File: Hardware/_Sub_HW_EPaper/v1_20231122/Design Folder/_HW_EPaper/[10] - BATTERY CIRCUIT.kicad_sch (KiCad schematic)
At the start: 0 parts

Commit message: Working on E-Paper schematic
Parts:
- added C1001, C1003: 1uF_10V_X7R, Capacitor_SMD:C_0402_1005Metric, symbol _SCHLIB_Epaper:CAP_1uF_10V_X7R_C0402
- added C1002, C1004: 100nF_50V, Capacitor_SMD:C_0402_1005Metric, symbol _SCHLIB_Epaper:CAP_100nF_50V_X7R_C0402
- added R1001: 10kR_1/16W_1%, Resistor_SMD:R_0402_1005Metric, symbol _SCHLIB_Epaper:RES_10kR_1/16W_1%_R0402
- added U1001: NCP551SN33T1G, Package_SO:TSOP-5_1.65x3.05mm_P0.95mm, symbol _SCHLIB_Epaper:PMIC_LDO_NCP551SN33T1G_+3V3DC_150mA_5-TSOP
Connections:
- new net: C1001.1, C1002.1, R1001.1, U1001.1 (VIN)
- new net +3V3: C1003.1, C1004.1, U1001.5 (VOUT)
- new net GND: C1001.2, C1002.2, C1003.2, C1004.2, U1001.2 (GND)
- new net NCP551_EN: R1001.2, U1001.3 (ENABLE)
- no-connect marks 0 -> 1

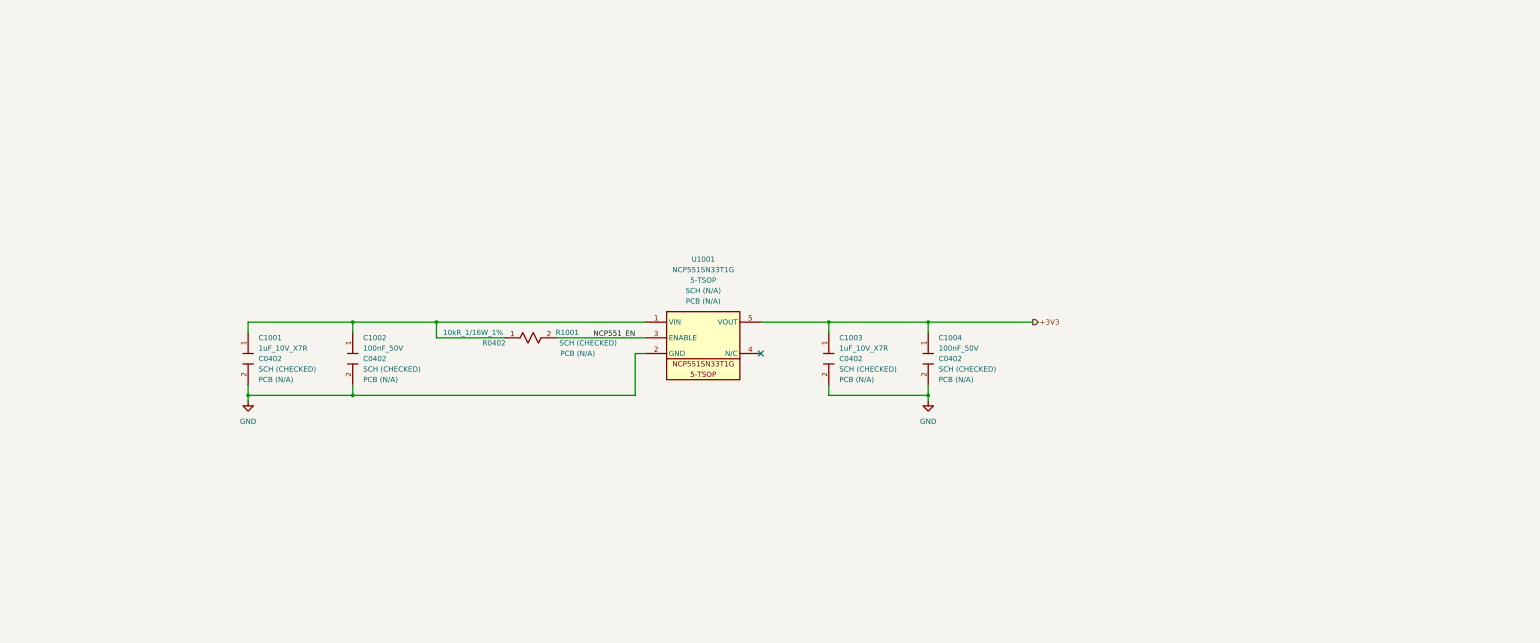
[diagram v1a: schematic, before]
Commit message: EPaper schematic is almost done...
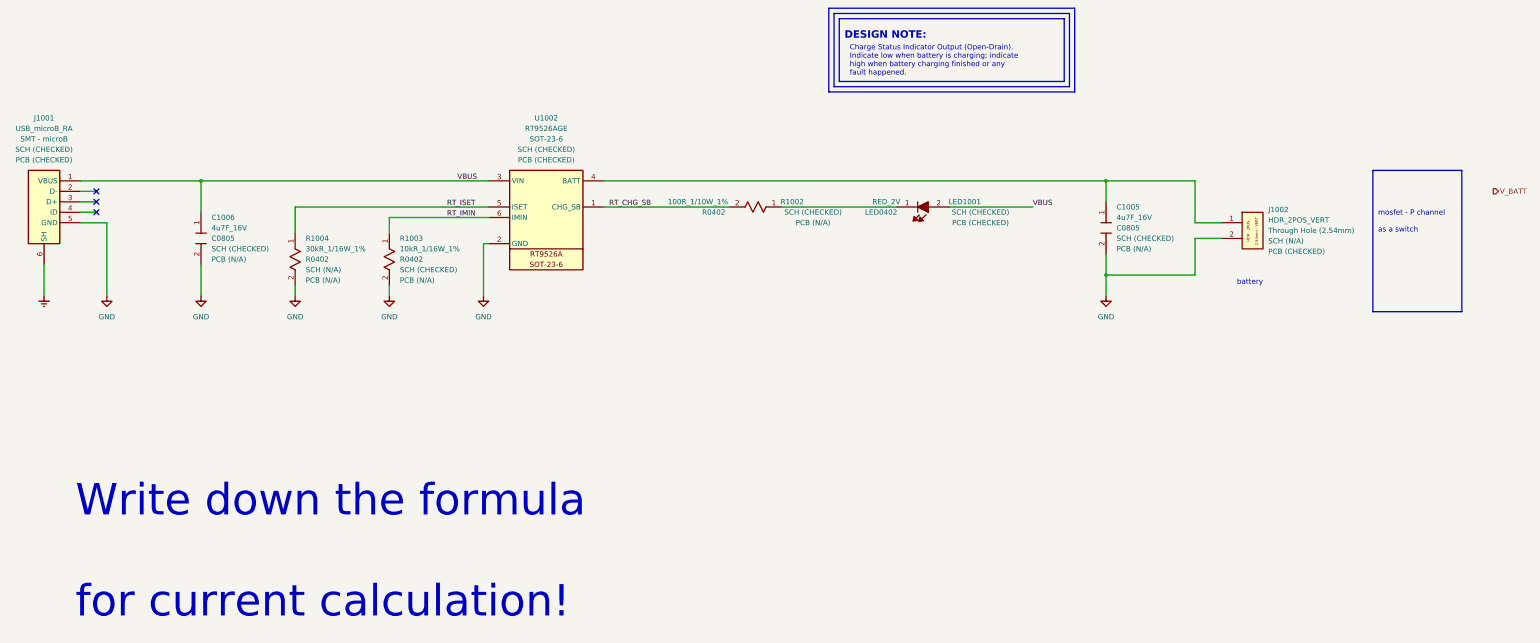
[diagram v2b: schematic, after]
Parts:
- removed C1001, C1003: 1uF_10V_X7R, Capacitor_SMD:C_0402_1005Metric, symbol _SCHLIB_Epaper:CAP_1uF_10V_X7R_C0402
- removed C1002, C1004: 100nF_50V, Capacitor_SMD:C_0402_1005Metric, symbol _SCHLIB_Epaper:CAP_100nF_50V_X7R_C0402
- removed R1001: 10kR_1/16W_1%, Resistor_SMD:R_0402_1005Metric, symbol _SCHLIB_Epaper:RES_10kR_1/16W_1%_R0402
- removed U1001: NCP551SN33T1G, Package_SO:TSOP-5_1.65x3.05mm_P0.95mm, symbol _SCHLIB_Epaper:PMIC_LDO_NCP551SN33T1G_+3V3DC_150mA_5-TSOP
- added C1005, C1006: 4u7F_16V, Capacitor_SMD:C_0805_2012Metric, symbol _SCHLIB_Epaper:CAP_4.7uF_16V_X7R_C0805
- added J1001: USB_microB_RA, Connector_USB:USB_Micro-B_Amphenol_10118194_Horizontal, symbol _SCHLIB_Epaper:CONN_RECEPT_USB2.0_microB_5POS_RA
- added J1002: HDR_2POS_VERT, Connector_PinHeader_2.54mm:PinHeader_1x02_P2.54mm_Vertical, symbol _SCHLIB_Epaper:CONN_HEADER_2POS_1ROW_VERT_2.54mm
- added LED1001: RED_2V, LED_SMD:LED_0402_1005Metric, symbol _SCHLIB_Epaper:LED_RED_2V_624nm_LED0402
- added R1002: 100R_1/10W_1%, Resistor_SMD:R_0402_1005Metric, symbol _SCHLIB_Epaper:RES_100R_1/10W_1%_R0402
- added R1003: 10kR_1/16W_1%, Resistor_SMD:R_0402_1005Metric, symbol _SCHLIB_Epaper:RES_10kR_1/16W_1%_R0402
- added R1004: 30kR_1/16W_1%, Resistor_SMD:R_0402_1005Metric, symbol _SCHLIB_Epaper:RES_30kR_1/16W_1%_R0402
- added U1002: RT9526AGE, Package_TO_SOT_SMD:SOT-23-6, symbol _SCHLIB_Epaper:PMIC_CHARGER_RT9526AGE_LithiumIon_1C_SOT-23-6
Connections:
- net GND: now also C1005.2, C1006.2, J1001.5 (GND), J1002.2, R1003.2, R1004.2, U1002.2 (GND)
- new net: C1005.1, J1002.1, U1002.4 (BATT)
- new net: LED1001.1, R1002.1
- new net Earth: J1001.6 (SH)
- new net RT_CHG_SB: R1002.2, U1002.1 (CHG_SB)
- new net RT_IMIN: R1003.1, U1002.6 (IMIN)
- new net RT_ISET: R1004.1, U1002.5 (ISET)
- new net VBUS: C1006.1, J1001.1 (VBUS), LED1001.2, U1002.3 (VIN)
- no-connect marks 1 -> 3
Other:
- note added: "Charge Status Indicator Output (Open-Drain). Indicate low when battery is charging; indicate high when battery charging finished or any fault happened."
- note added: "DESIGN NOTE:"
- note added: "Write down the formula for current calculation!"
- note added: "battery"
- note added: "mosfet - P channel as a switch"

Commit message: Latest update
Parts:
- added D1001: TVS_6.5V_3A, _PCBLIB_Epaper:CR_7PCT_L3F_TOS, symbol _SCHLIB_Epaper:TVS_5V(MAX)_6.5(Vbr-min)_3A(8/20us)_SOD882
- added F1001: 100mA_15V_0.5R, Fuse:Fuse_0603_1608Metric, symbol _SCHLIB_Epaper:FUSE_100mA(Ih)_250mA(It)_15V_0.5Ohm_F0603
- added Q1001: SSM3J117TU,LF, _PCBLIB_Epaper:UFM_TOS, symbol _SCHLIB_Epaper:Q_P-Channel_30V_2A_SSM3J117TU,LF_UFM
- added R1001: 10kR_1/16W_1%, Resistor_SMD:R_0402_1005Metric, symbol _SCHLIB_Epaper:RES_10kR_1/16W_1%_R0402
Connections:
- net GND: now also D1001.2, R1001.2
- net VBUS: now also D1001.1, F1001.2, Q1001.1, R1001.1; no longer J1001.1 (VBUS)
- net V_BATT: now also Q1001.3
- net RT_BATT: now reaches C1005.1, J1002.1, U1002.4 (BATT)
- net RT_BATT: now also Q1001.2
- new net: F1001.1, J1001.1 (VBUS)
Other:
- note added: "Battery connector"
- note added: "INFO:"
- note removed: "battery"
- note removed: "mosfet - P channel as a switch"
- moved on the sheet: C1005, C1006, J1001, J1002, LED1001, R1002, R1003, R1004, U1002

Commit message: Working on epaper hardware
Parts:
- added R703: 470R_1/16W_1%, Resistor_SMD:R_0402_1005Metric, symbol _SCHLIB_Epaper:RES_470R_1/16W_1%_R0402
- renumbered C1005 to C1001, C1006 to C1002, R1002 to R1001, R1004 to R1002, R1001 to R1005, U1002 to U1001
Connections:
- net VBUS: now also R703.1; no longer Q1001.1, R1005.1
- new net: Q1001.1, R1005.1, R703.2
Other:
- note added: "Battery Fast-Charge Current ICHG_FAST = KISET x VISET/RISET KSET = 9959R; VSET = 1.22V ICHG_FAST = (9959 * 1.22) / 30000 = 404 mA"
- note added: "End-Of-Charge Current (EOC) IMIN = 10935/RIMIN = 10935/10000 = 1.0935 mA"
- note added: "LAYOUT NOTE:"
- note removed: "Write down the formula for current calculation!"
- moved on the sheet: C1001, C1002, D1001, F1001, J1001, J1002, LED1001, Q1001, R1001, R1002, R1003, R1005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

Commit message: Hardware is almost done
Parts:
- J1001: footprint Connector_USB:USB_Micro-B_Amphenol_10118194_Horizontal -> _PCBLIB_Epaper:USB_Micro-B_Amphenol_10118194_Horizontal
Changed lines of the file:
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@@
       (effects (font (size 1.27 1.27)))
     )
-    (property "Footprint" "Connector_USB:USB_Micro-B_Amphenol_10118194_Horizontal" (at 24.13 83.82 0)
+    (property "Footprint" "_PCBLIB_Epaper:USB_Micro-B_Amphenol_10118194_Horizontal" (at 24.13 83.82 0)
       (effects (font (size 1.27 1.27)) (justify left) hide)
     )

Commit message: Updating file templates and structures...
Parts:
- C1001, C1002: Manufacturer (none) -> Murata Electronics; Part Number GRM21BR71C475KE51L -> (none); Part Number (Manufacturer) (none) -> GRM21BR71C475KE51L; Part Number (Vendor) (none) -> 490-14466-2-ND; Vendor (none) -> Digikey
- D1001: Manufacturer (none) -> Good-Ark Semiconductor; Part Number GSEWT5B003 -> (none); Part Number (Manufacturer) (none) -> GSEWT5B003; Part Number (Vendor) (none) -> 4786-GSEWT5B003TR-ND; Vendor (none) -> Digikey
- F1001: Manufacturer (none) -> Eaton - Electronics Division; Part Number PTS060315V010 -> (none); Part Number (Manufacturer) (none) -> PTS060315V010; Part Number (Vendor) (none) -> 283-PTS060315V010TR-ND; Vendor (none) -> Digikey
- J1001: Manufacturer (none) -> Adam Tech; Part Number 10118194-0001LF -> (none); Part Number (Manufacturer) (none) -> 10118194-0001LF; Part Number (Vendor) (none) -> 2057-PH1RB-08-UA-ND; Vendor (none) -> Digikey
- J1002: Manufacturer (none) -> Adam Tech; Part Number PH1-02-UA -> (none); Part Number (Manufacturer) (none) -> PH1-02-UA; Part Number (Vendor) (none) -> 2057-PH1-02-UA-ND; Vendor (none) -> Digikey
- LED1001: Manufacturer (none) -> Harvatek Corporation; Part Number B2841USD-20D001014U1930 -> (none); Part Number (Manufacturer) (none) -> B2841USD-20D001014U1930; Part Number (Vendor) (none) -> 3147-B2841USD-20D001014U1930TR-ND; Vendor (none) -> Digikey
- Q1001: Manufacturer (none) -> Toshiba Semiconductor and Storage; Part Number SSM3J117TU,LF -> (none); Part Number (Manufacturer) (none) -> SSM3J117TU,LF; Part Number (Vendor) (none) -> SSM3J117TULFTR-ND; Vendor (none) -> Digikey
- R1001: Manufacturer (none) -> KOA Speer Electronics, Inc.; Part Number RK73H1ETTP1000F -> (none); Part Number (Manufacturer) (none) -> RK73H1ETTP1000F; Part Number (Vendor) (none) -> 2019-RK73H1ETTP1000FTR-ND; Vendor (none) -> Digikey
- R1002: Manufacturer (none) -> Bourns Inc.; Part Number CR0402-FX-3002GLF -> (none); Part Number (Manufacturer) (none) -> CR0402-FX-3002GLF; Part Number (Vendor) (none) -> CR0402-FX-3002GLFTR-ND; Vendor (none) -> Digikey
- R1003, R1005: Manufacturer (none) -> Bourns Inc.; Part Number CR0402-FX-1002GLF -> (none); Part Number (Manufacturer) (none) -> CR0402-FX-1002GLF; Part Number (Vendor) (none) -> CR0402-FX-1002GLFTR-ND; Vendor (none) -> Digikey
- R703: Manufacturer (none) -> Bourns Inc.; Part Number CR0402-FX-4700GLF -> (none); Part Number (Manufacturer) (none) -> CR0402-FX-4700GLF; Part Number (Vendor) (none) -> CR0402-FX-4700GLFTR-ND; Vendor (none) -> Digikey
- U1001: Manufacturer (none) -> Richtek USA Inc.; Part Number RT9526AGE -> (none); Part Number (Manufacturer) (none) -> RT9526AGE; Part Number (Vendor) (none) -> 1028-1359-2-ND; Vendor (none) -> Digikey
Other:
- moved on the sheet: C1001, C1002, D1001, F1001, J1001, J1002, LED1001, Q1001, R1001, R1002, R1003, R1005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
